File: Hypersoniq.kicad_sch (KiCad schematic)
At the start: 33 parts, among them J1 Conn_01x10_Pin, J2 Conn_01x10_Pin, J3 Conn_01x10_Pin, J4 Eurorack_10_pin_power, U1 TL074, U6 TL072

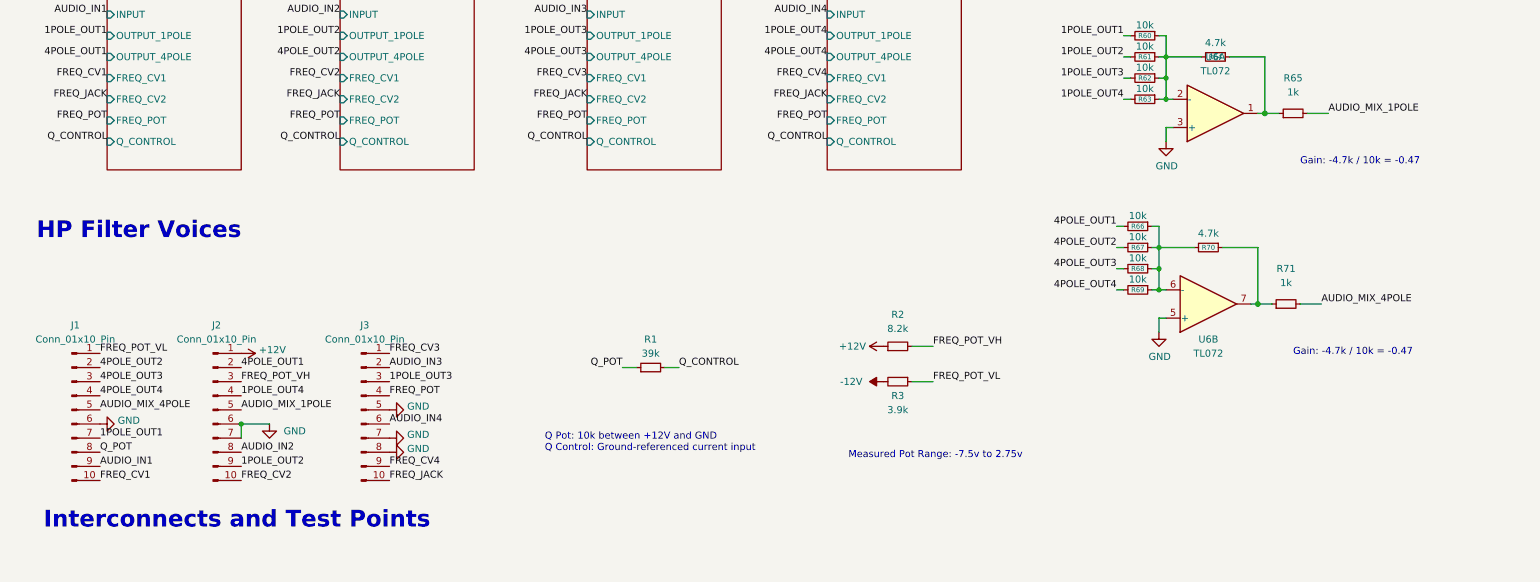
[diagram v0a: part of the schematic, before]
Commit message: Revert "PCB Layout"
This reverts commit f9e64c4088f3b37948fb3949196b7229d7a48ca0.
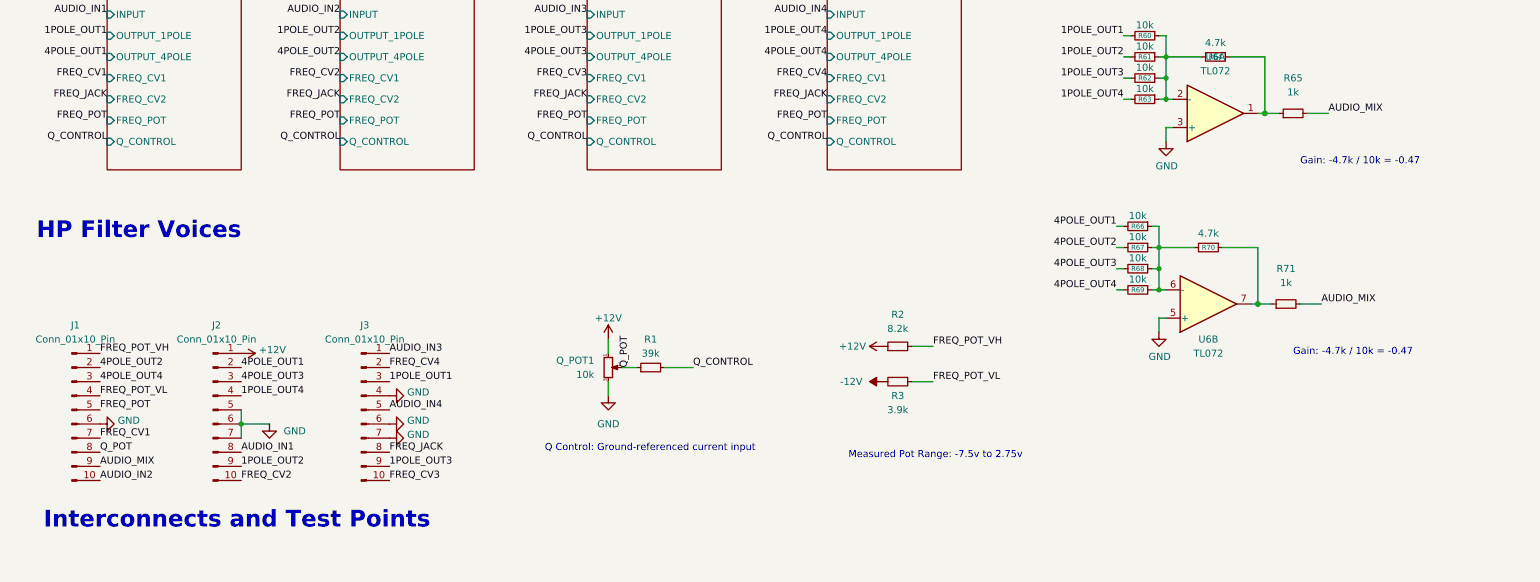
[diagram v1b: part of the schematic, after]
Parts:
- added Q_POT1: 10k, Custom_Footprints:Alpha_9mm_Potentiometer_Aligned, symbol Device:R_Potentiometer_Small
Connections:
- net +12V: now also Q_POT1.1
- net 1POLE_OUT1: now also J3.3 (Pin_3); no longer J1.7 (Pin_7)
- net 1POLE_OUT3: now also J3.9 (Pin_9); no longer J3.3 (Pin_3)
- net 4POLE_OUT3: now also J2.3 (Pin_3); no longer J1.3 (Pin_3)
- net 4POLE_OUT4: now also J1.3 (Pin_3); no longer J1.4 (Pin_4)
- net AUDIO_IN1: now also J2.8 (Pin_8); no longer J1.9 (Pin_9)
- net AUDIO_IN2: now also J1.10 (Pin_10); no longer J2.8 (Pin_8)
- net AUDIO_IN3: now also J3.1 (Pin_1); no longer J3.2 (Pin_2)
- net AUDIO_IN4: now also J3.5 (Pin_5); no longer J3.6 (Pin_6)
- net FREQ_CV1: now also J1.7 (Pin_7); no longer J1.10 (Pin_10)
- net FREQ_CV3: now also J3.10 (Pin_10); no longer J3.1 (Pin_1)
- net FREQ_CV4: now also J3.2 (Pin_2); no longer J3.9 (Pin_9)
- net FREQ_JACK: now also J3.8 (Pin_8); no longer J3.10 (Pin_10)
- net FREQ_POT: now also J1.5 (Pin_5); no longer J3.4 (Pin_4)
- net FREQ_POT_VH: now also J1.1 (Pin_1); no longer J2.3 (Pin_3)
- net FREQ_POT_VL: now also J1.4 (Pin_4); no longer J1.1 (Pin_1)
- net GND: now also J2.5 (Pin_5), J3.4 (Pin_4), J3.6 (Pin_6), Q_POT1.3; no longer J3.5 (Pin_5), J3.8 (Pin_8)
- net Q_POT: now also Q_POT1.2
- net AUDIO_MIX_1POLE renamed AUDIO_MIX
- net AUDIO_MIX: now also J1.9 (Pin_9), R71.2; no longer J2.5 (Pin_5)
- removed net AUDIO_MIX_4POLE: J1.5 (Pin_5), R71.2
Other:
- note added: "Q Control: Ground-referenced current input"
- note removed: "Q Pot: 10k between +12V and GND Q Control: Ground-referenced current input"
